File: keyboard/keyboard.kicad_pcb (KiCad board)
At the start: 2 copper layers, 127.1 x 77.5 mm, 21 parts

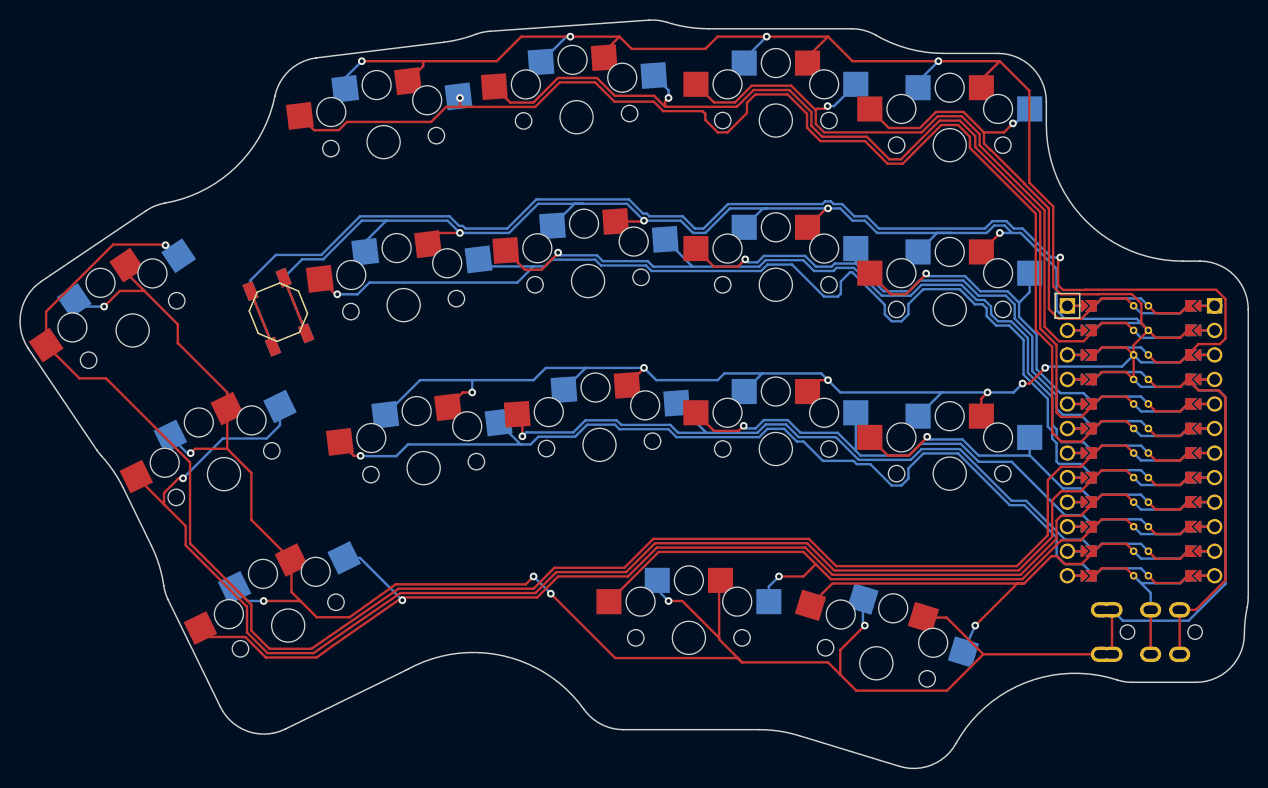
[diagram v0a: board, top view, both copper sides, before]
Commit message: Tent puck and some cleanup
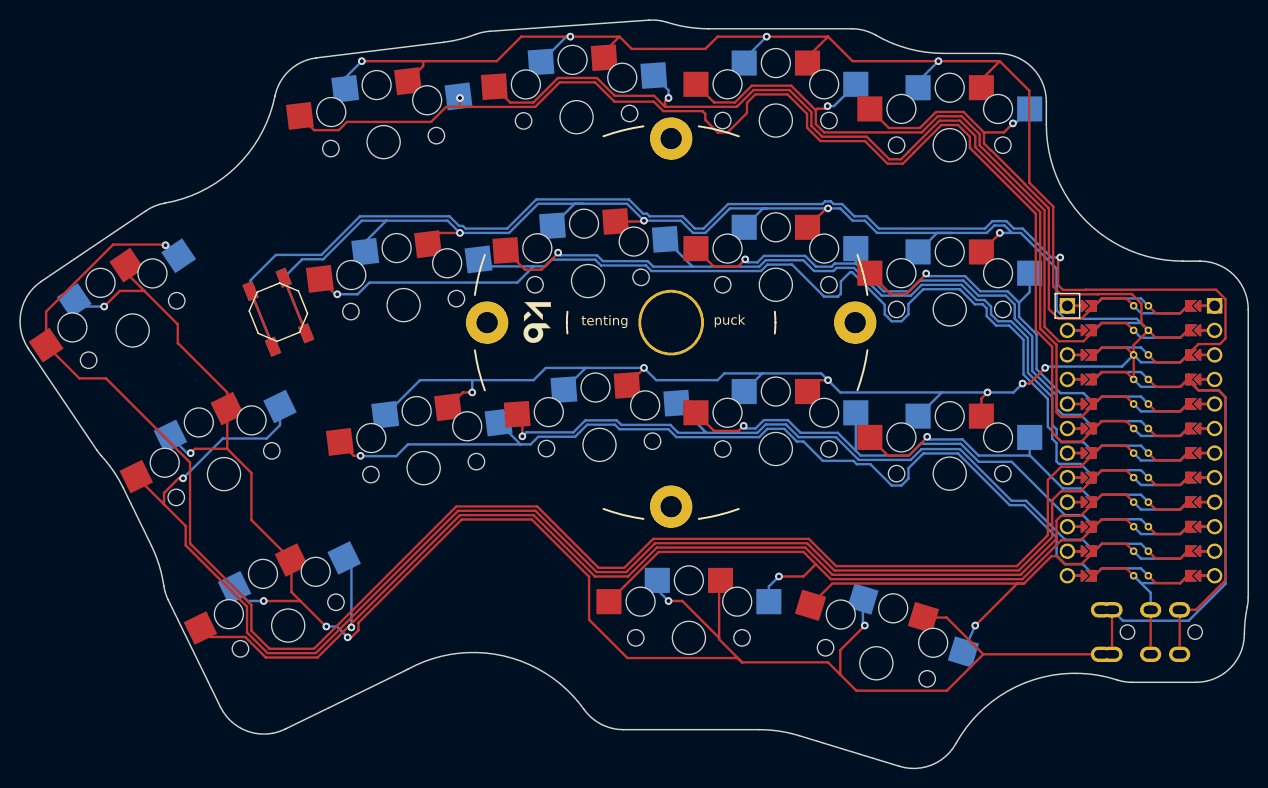
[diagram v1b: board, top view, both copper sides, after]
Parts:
- added REF**: Tenting Puck, Library:TentingPuck, F.Cu at (39.6, -31.4)
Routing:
- net GND: track 617.6 -> 627.6 mm
- net main_pinkie_top: track 162.0 -> 167.9 mm
- net main_pinkie_home: track 139.0 -> 144.9 mm
- net main_pinkie_bottom: track 111.4 -> 115.9 mm
